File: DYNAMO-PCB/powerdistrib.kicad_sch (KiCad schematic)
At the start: 10 parts, among them J17 USB3_A, J19 USB3_A, J2 USB3_A, J20 USB3_A, J26 USB_C_Receptacle_USB2.0_16P, J27 USB_C_Receptacle_USB2.0_16P, J28 USB_C_Receptacle_USB2.0_16P, J30 USB_C_Receptacle_USB2.0_16P

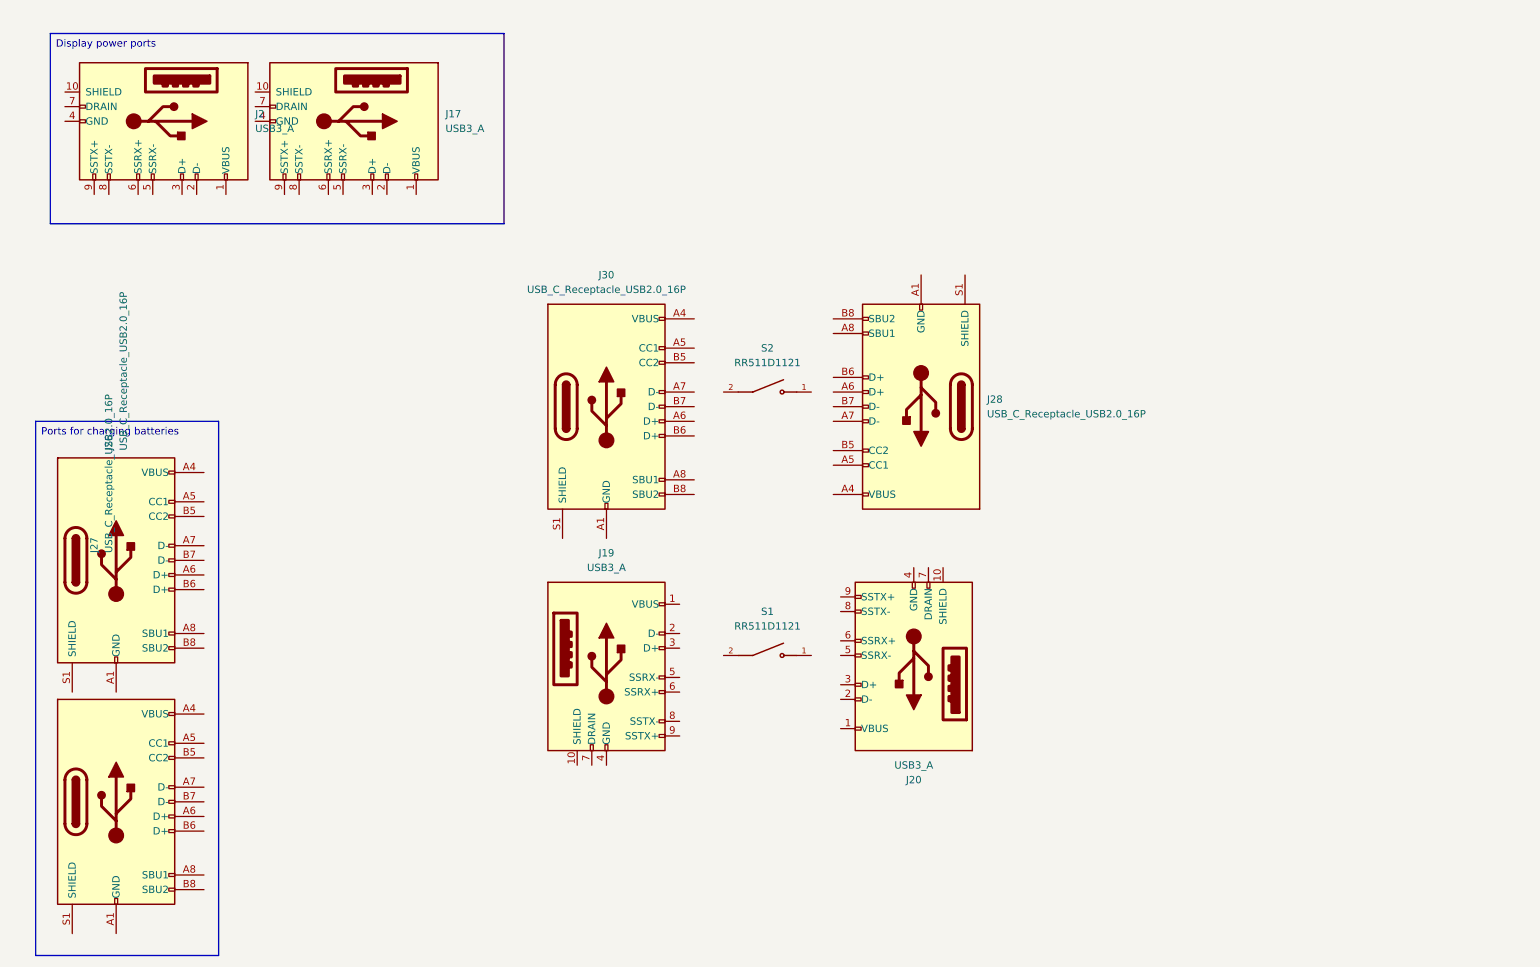
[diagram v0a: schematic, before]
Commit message: schematic wip
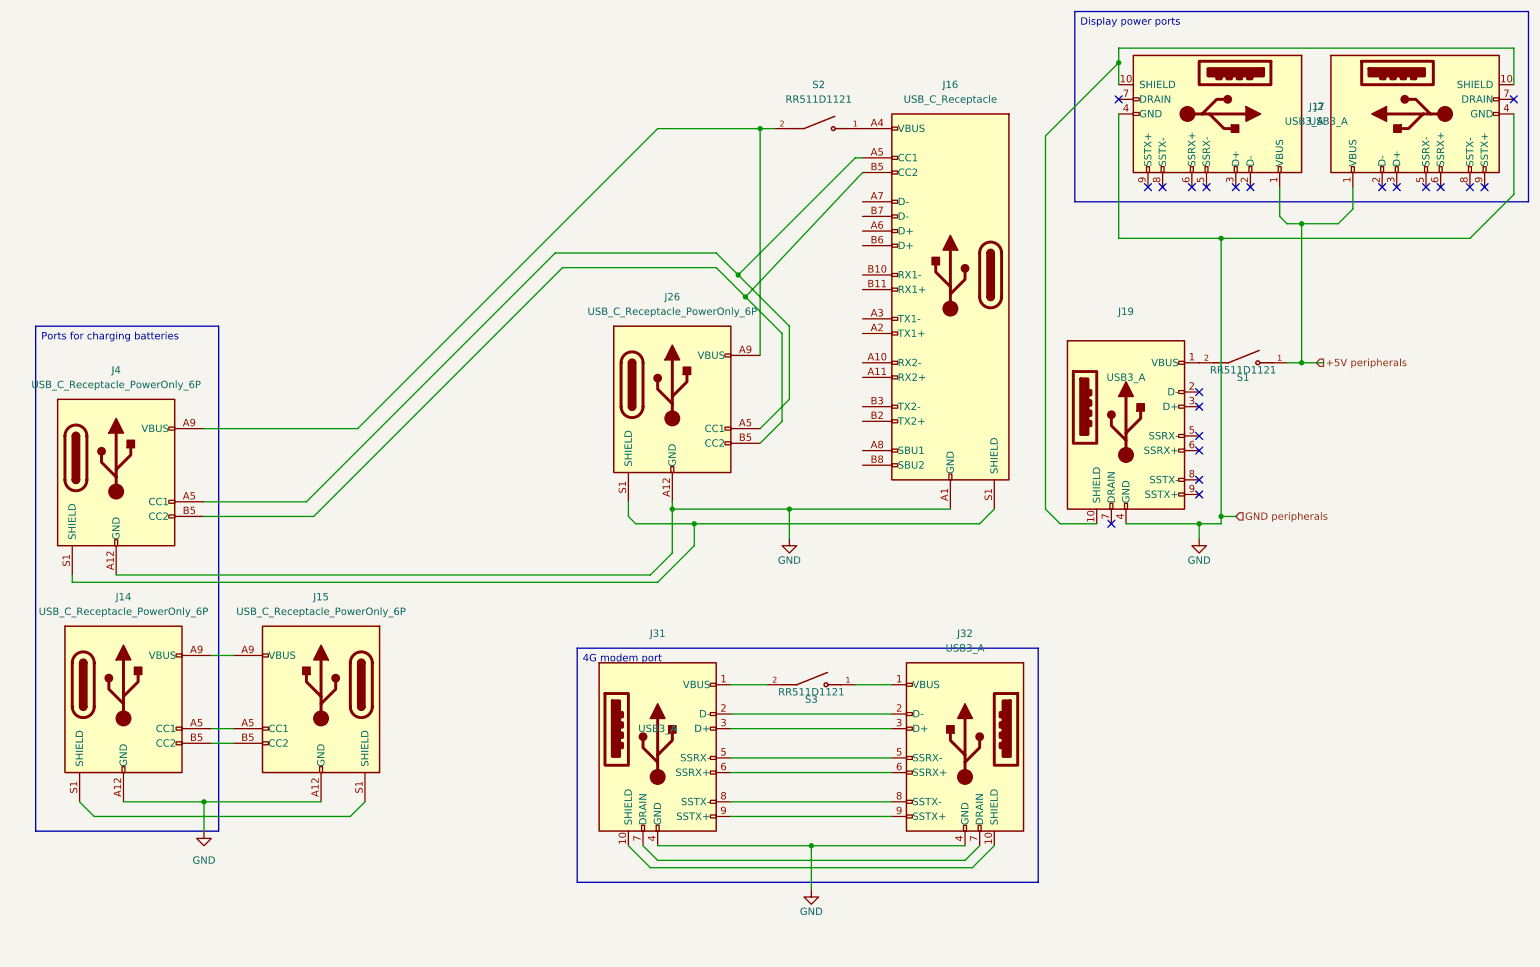
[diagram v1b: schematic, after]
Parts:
- removed J20: USB3_A, 692122030100:692122030100, symbol Connector:USB3_A
- removed J26, J27, J28, J30: USB_C_Receptacle_USB2.0_16P, Connector_USB:USB_C_Receptacle_GCT_USB4105-xx-A_16P_TopMnt_Horizontal, symbol Connector:USB_C_Receptacle_USB2.0_16P
- added J14, J15, J26, J4: USB_C_Receptacle_PowerOnly_6P, symbol Connector:USB_C_Receptacle_PowerOnly_6P
- added J16: USB_C_Receptacle, symbol Connector:USB_C_Receptacle
- added J31, J32: USB3_A, 692122030100:692122030100, symbol Connector:USB3_A
- added S3: RR511D1121, RR511D1121:E-SWITCH_RR511D1121, symbol RR511D1121:RR511D1121
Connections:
- net +5V peripherals: now reaches S1.1
- net +5V peripherals: now also J17.1 (VBUS), J2.1 (VBUS)
- net at S1.2: now also J19.1 (VBUS)
- net at J19.10 (SHIELD): now also J17.10 (SHIELD), J2.10 (SHIELD)
- net GND: now reaches J19.4 (GND)
- net GND: now also J17.4 (GND), J2.4 (GND), J14.A12 (GND), J14.B12 (GND), J15.A12 (GND), J15.B12 (GND), J16.A1 (GND), J16.A12 (GND), J16.B1 (GND), J16.B12 (GND), J26.A12 (GND), J26.B12 (GND), J31.4 (GND), J32.4 (GND), J4.A12 (GND), J4.B12 (GND)
- net at S2.1: now also J16.A4 (VBUS), J16.A9 (VBUS), J16.B4 (VBUS), J16.B9 (VBUS)
- net at S2.2: now also J26.A9 (VBUS), J26.B9 (VBUS), J4.A9 (VBUS), J4.B9 (VBUS)
- new net: J14.A5 (CC1), J15.A5 (CC1)
- new net: J14.A9 (VBUS), J14.B9 (VBUS), J15.A9 (VBUS), J15.B9 (VBUS)
- new net: J14.B5 (CC2), J15.B5 (CC2)
- new net: J14.S1 (SHIELD), J15.S1 (SHIELD)
- new net: J16.A5 (CC1), J26.A5 (CC1), J4.A5 (CC1)
- new net: J16.B5 (CC2), J26.B5 (CC2), J4.B5 (CC2)
- new net: J16.S1 (SHIELD), J26.S1 (SHIELD), J4.S1 (SHIELD)
- new net: J31.1 (VBUS), S3.2
- new net: J31.10 (SHIELD), J32.10 (SHIELD)
- new net: J31.2 (D-), J32.2 (D-)
- new net: J31.3 (D+), J32.3 (D+)
- new net: J31.5 (SSRX-), J32.5 (SSRX-)
- new net: J31.6 (SSRX+), J32.6 (SSRX+)
- new net: J31.7 (DRAIN), J32.7 (DRAIN)
- new net: J31.8 (SSTX-), J32.8 (SSTX-)
- new net: J31.9 (SSTX+), J32.9 (SSTX+)
- new net: J32.1 (VBUS), S3.1
- no-connect marks 0 -> 21
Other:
- moved on the sheet: J17, J19, J2, S1, S2
